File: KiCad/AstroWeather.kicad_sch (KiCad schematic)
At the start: 8 parts, among them J101 USB_C_Receptacle_USB2.0_14P, J102 Conn_01x10, J103 Conn_01x10, J104 AUX_POWER, J105 SWD, J106 I2C

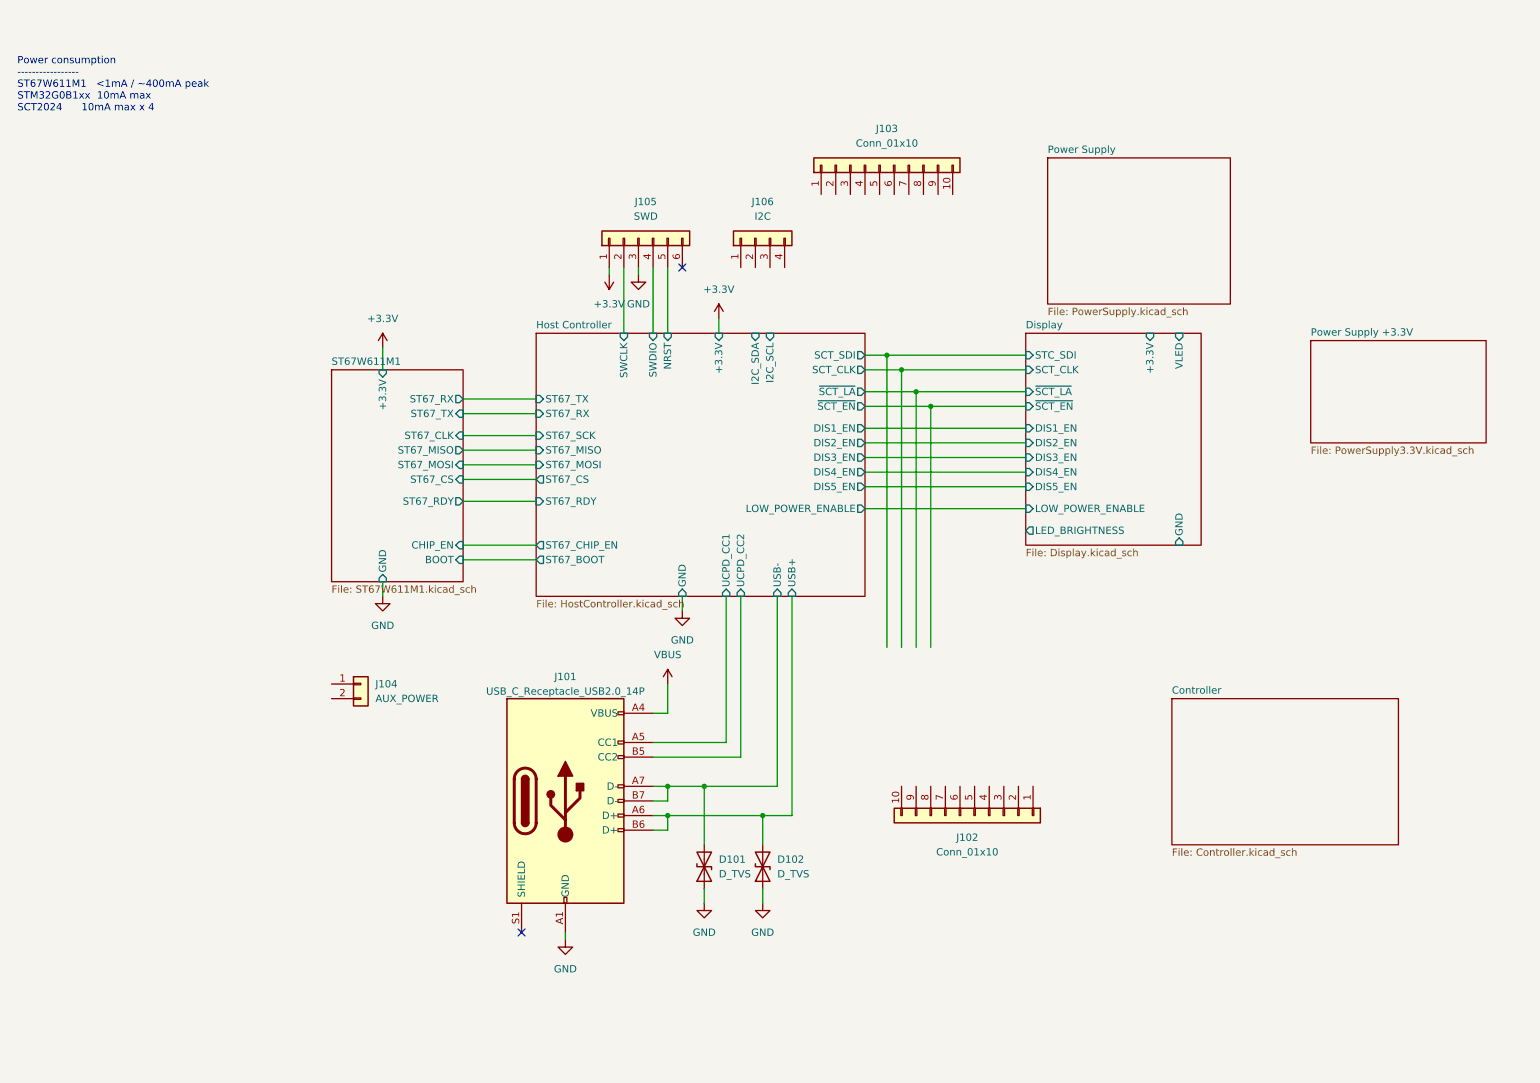
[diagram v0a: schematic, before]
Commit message: KiCad work
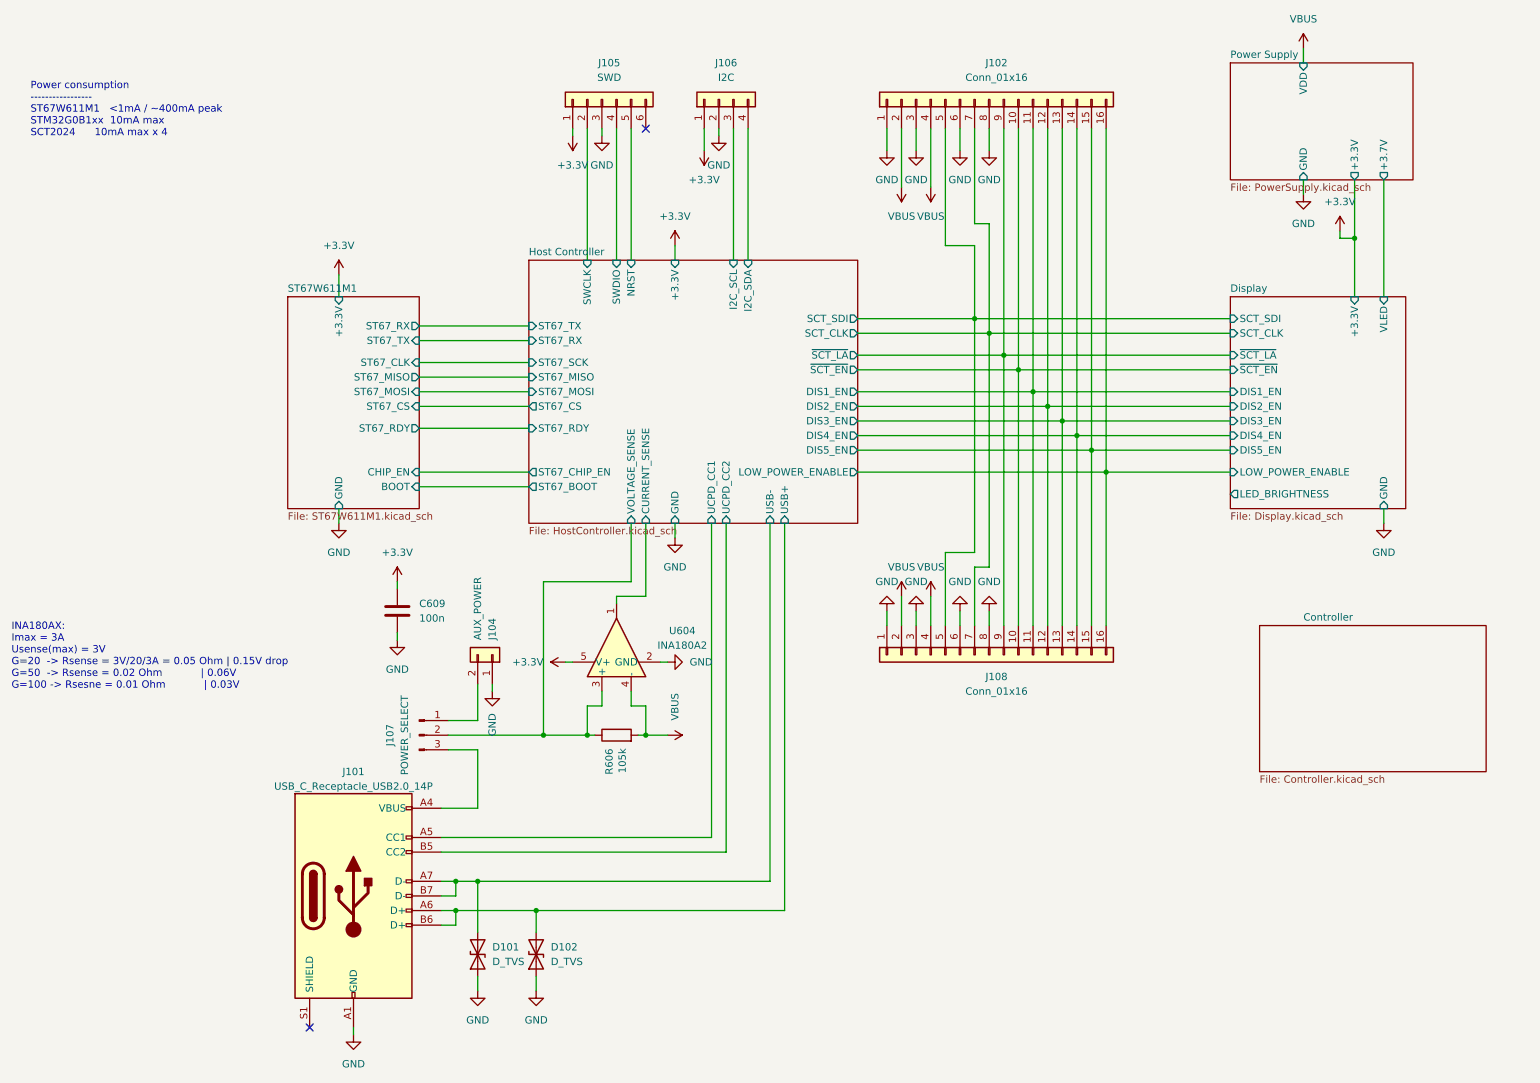
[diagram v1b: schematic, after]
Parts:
- removed J102, J103: Conn_01x10, symbol Connector_Generic:Conn_01x10
- added C609: 100n, symbol Device:C
- added J102, J108: Conn_01x16, symbol Connector_Generic:Conn_01x16
- added J107: POWER_SELECT, symbol Connector:Conn_01x03_Pin
- added R606: 105k, symbol Device:R
- added U604: INA180A2, Package_TO_SOT_SMD:SOT-23-5, symbol Amplifier_Current:INA180A2
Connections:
- net +3.3V: now also J106.1 (Pin_1), C609.1, U604.5 (V+)
- net Display/DIS1_EN: now also J102.11 (Pin_11), J108.11 (Pin_11)
- net Display/DIS2_EN: now also J102.12 (Pin_12), J108.12 (Pin_12)
- net Display/DIS3_EN: now also J102.13 (Pin_13), J108.13 (Pin_13)
- net Display/DIS4_EN: now also J102.14 (Pin_14), J108.14 (Pin_14)
- net Display/DIS5_EN: now also J102.15 (Pin_15), J108.15 (Pin_15)
- net Display/LOW_POWER_ENABLE: now also J102.16 (Pin_16), J108.16 (Pin_16)
- net Display/SCT_CLK: now also J102.7 (Pin_7), J108.7 (Pin_7)
- net Display/~{SCT_EN}: now also J102.10 (Pin_10), J108.10 (Pin_10)
- net Display/~{SCT_LA}: now also J102.9 (Pin_9), J108.9 (Pin_9)
- net GND: now also J104.1 (Pin_1), J106.2 (Pin_2), C609.2, J102.1 (Pin_1), J102.3 (Pin_3), J102.6 (Pin_6), J102.8 (Pin_8), J108.1 (Pin_1), J108.3 (Pin_3), J108.6 (Pin_6), J108.8 (Pin_8), U604.2 (GND)
- net Host Controller/I2C_SCL: now also J106.3 (Pin_3)
- net Host Controller/I2C_SDA: now also J106.4 (Pin_4)
- net VBUS: now also J102.2 (Pin_2), J102.4 (Pin_4), J108.2 (Pin_2), J108.4 (Pin_4), R606.2, U604.4 (-); no longer J101.A4 (VBUS), J101.A9 (VBUS), J101.B4 (VBUS), J101.B9 (VBUS)
- net at J104.2 (Pin_2): now also J107.1 (Pin_1)
- new net: J101.A4 (VBUS), J101.A9 (VBUS), J101.B4 (VBUS), J101.B9 (VBUS), J107.3 (Pin_3)
- new net Display/SCT_SDI: J102.5 (Pin_5), J108.5 (Pin_5)
- new net Host Controller/CURRENT_SENSE: U604.1
- new net Host Controller/VOLTAGE_SENSE: J107.2 (Pin_2), R606.1, U604.3 (+)
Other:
- removed sheet Power Supply +3.3V
- sheet Display ports: added SCT_SDI; removed STC_SDI
- sheet Host Controller ports: added CURRENT_SENSE, VOLTAGE_SENSE; removed none
- sheet Power Supply ports: added +3.3V, +3.7V, GND, VDD; removed none
- note added: "INA180AX: Imax = 3A Usense(max) = 3V G=20 -> Rsense = 3V/20/3A = 0.05 Ohm | 0.15V drop G=50 -> Rsense = 0.02 Ohm | 0.06V G=100 -> Rsesne = 0.01 Ohm | 0.03V"
- moved on the sheet: D101, D102, J101, J104, J105, J106
